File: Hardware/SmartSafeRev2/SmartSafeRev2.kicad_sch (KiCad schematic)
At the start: 15 parts

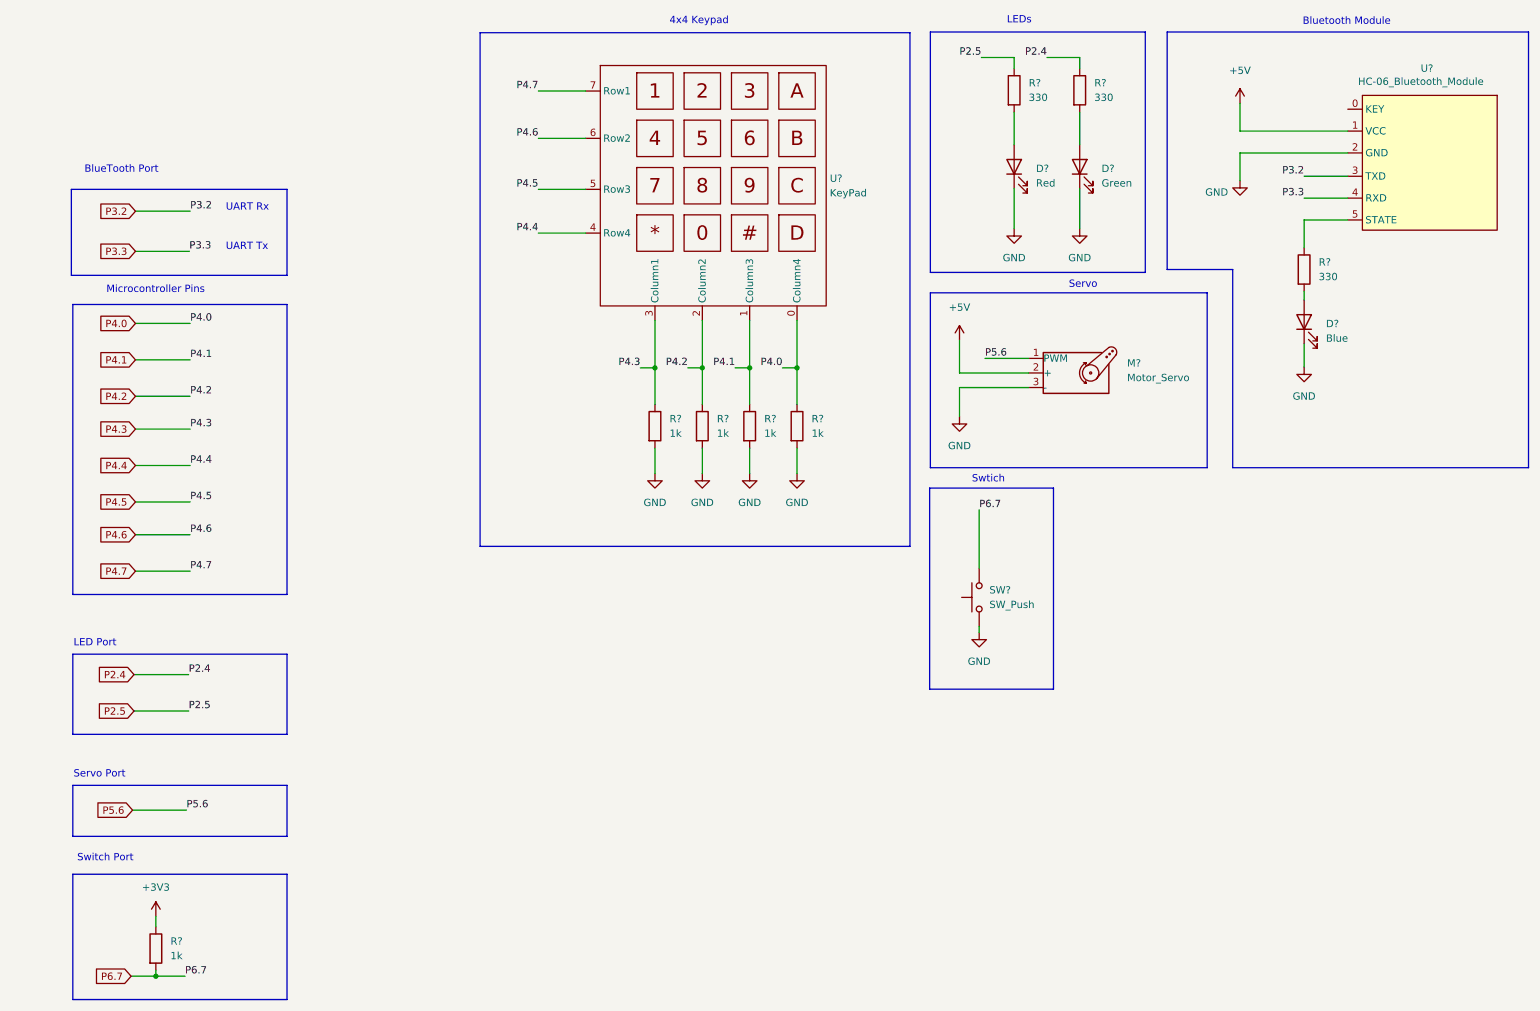
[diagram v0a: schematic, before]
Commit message: Schematic update
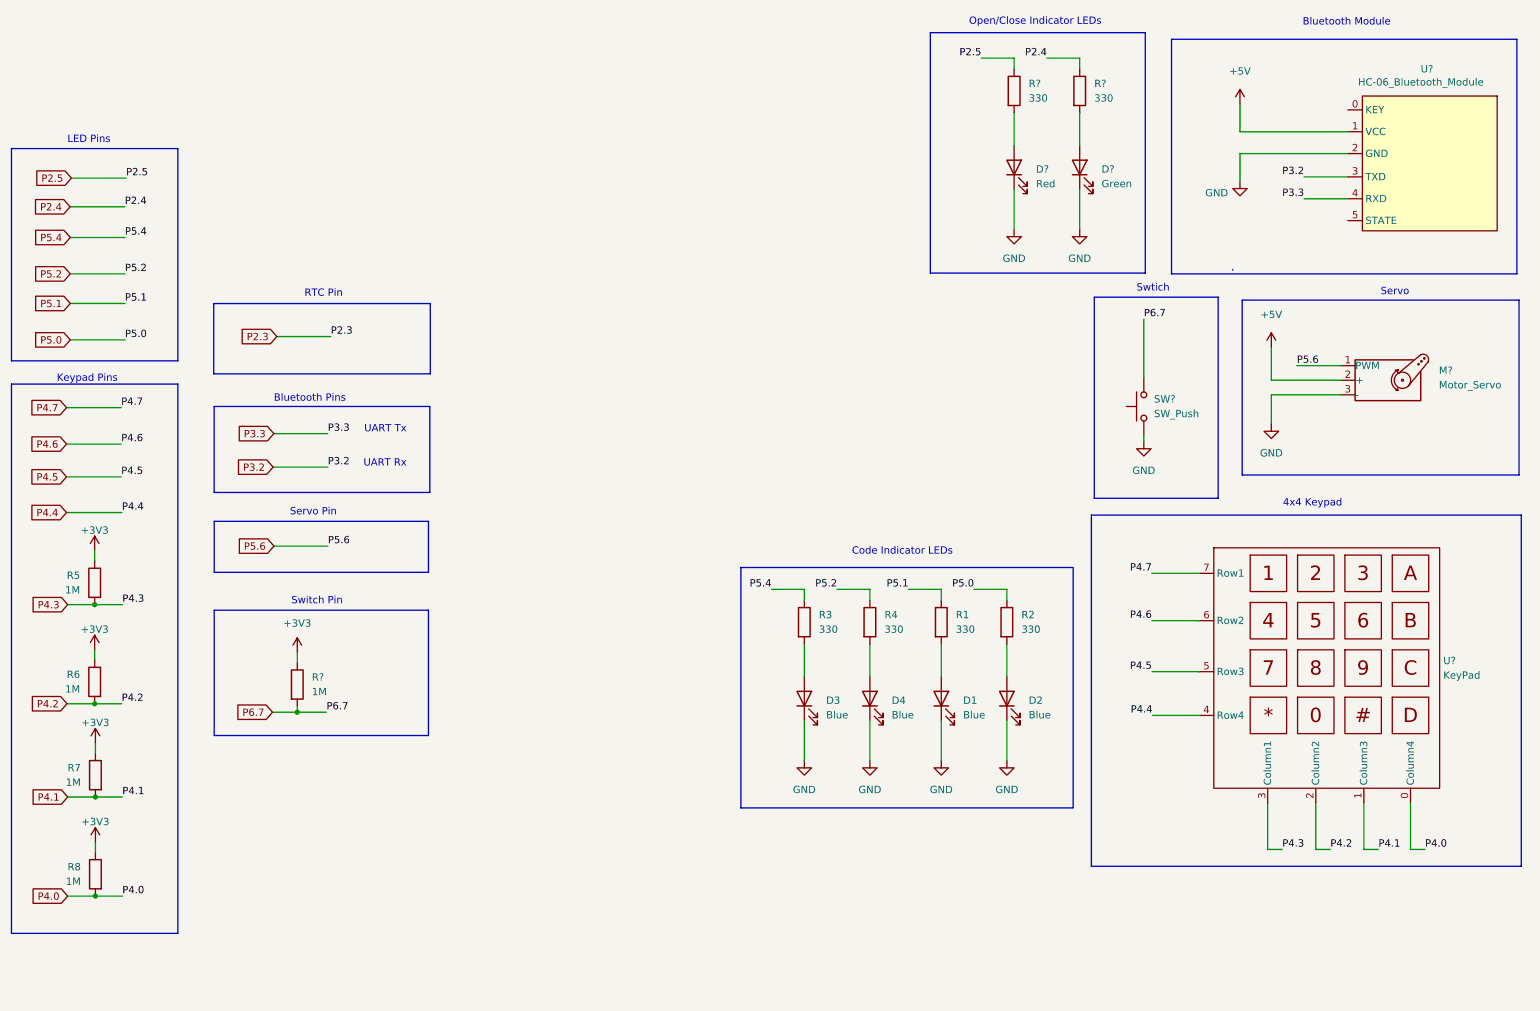
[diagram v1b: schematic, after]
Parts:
- removed D?: Blue, symbol Device:LED
- removed R? (x4): 1k, symbol Device:R
- removed R?: 330, symbol Device:R
- added D1, D2, D3, D4: Blue, symbol Device:LED
- added R1, R2, R3, R4: 330, symbol Device:R
- added R5, R6, R7, R8: 1M, symbol Device:R
- R?: value 1k -> 1M
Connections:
- net +3V3: now also R5.1, R6.1, R7.1, R8.1
- net GND: now also D1.1 (K), D2.1 (K), D3.1 (K), D4.1 (K)
- net P4.0: now also R8.2
- net P4.1: now also R7.2
- net P4.2: now also R6.2
- net P4.3: now also R5.2
- new net: D1.2 (A), R1.2
- new net: D2.2 (A), R2.2
- new net: D4.2 (A), R4.2
- new net: D3.2 (A), R3.2
- new net P5.0: R2.1
- new net P5.1: R1.1
- new net P5.2: R4.1
- new net P5.4: R3.1
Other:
- note added: "Bluetooth Pins"
- note added: "Code Indicator LEDs"
- note added: "Keypad Pins"
- note added: "LED Pins"
- note added: "Open/Close Indicator LEDs"
- note added: "RTC Pin"
- note added: "Servo Pin"
- note added: "Switch Pin"
- note removed: "BlueTooth Port"
- note removed: "LED Port"
- note removed: "LEDs"
- note removed: "Microcontroller Pins"
- note removed: "Servo Port"
- note removed: "Switch Port"
- moved on the sheet: M?, R?, SW?, U?
